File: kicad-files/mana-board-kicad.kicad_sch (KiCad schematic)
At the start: 39 parts, among them U1 Pico

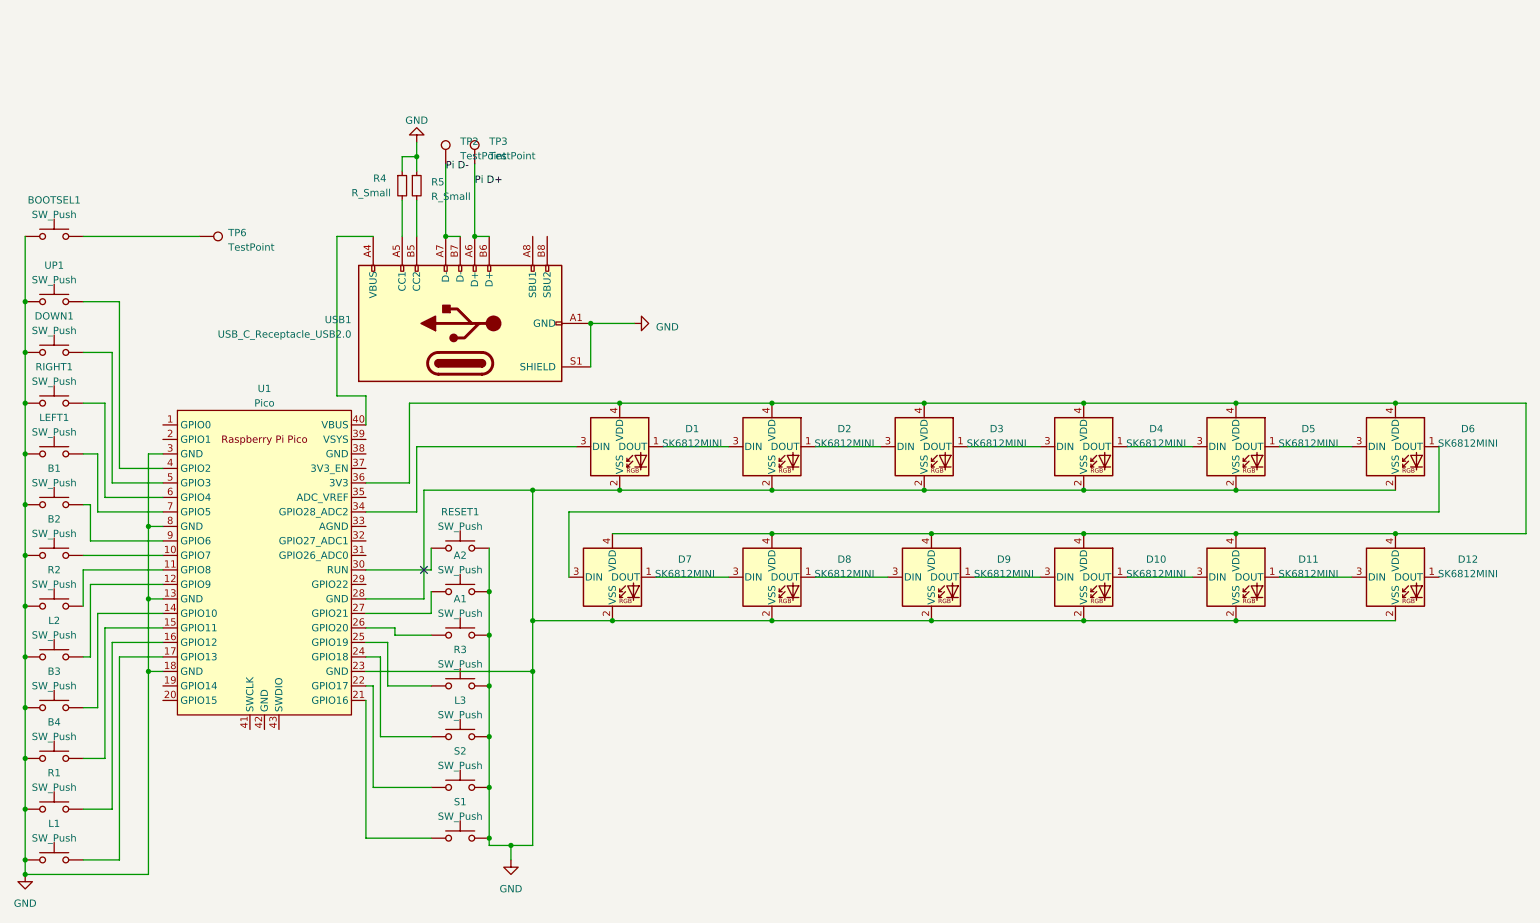
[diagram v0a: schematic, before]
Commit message: Organize libraries, start rev1
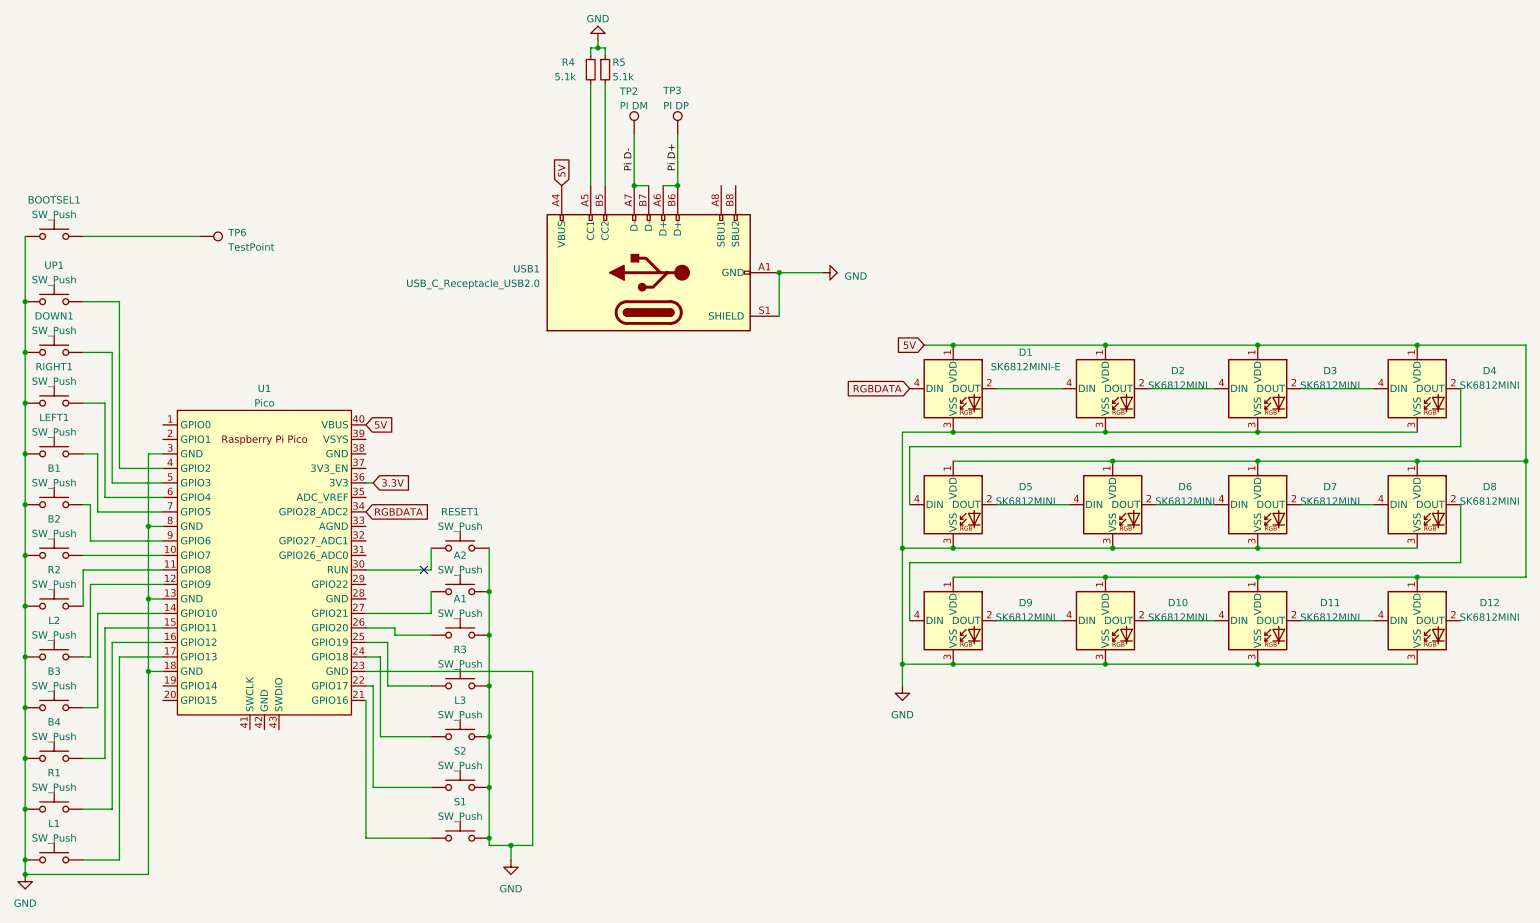
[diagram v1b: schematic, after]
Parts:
- D1: value SK6812MINI -> SK6812MINI-E; footprint Footprints:SK6812-MINI-E-reversed -> Keebio-Parts:SK6812-MINI-E; symbol LED:SK6812MINI -> ManaBoard:SK6812MINI-E
- D10, D11, D12, D2, D3, D4, D5, D6, D7, D8, D9: footprint Footprints:SK6812-MINI-E-reversed -> Keebio-Parts:SK6812-MINI-E; symbol LED:SK6812MINI -> ManaBoard:SK6812MINI-E
- R4, R5: value R_Small -> 5.1k
- TP2: value TestPoint -> PI DM
- TP3: value TestPoint -> PI DP
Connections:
- net GND: now also D1.3 (VSS), D10.3 (VSS), D11.3 (VSS), D12.3 (VSS), D2.3 (VSS), D3.3 (VSS), D4.3 (VSS), D5.3 (VSS), D6.3 (VSS), D7.3 (VSS), D8.3 (VSS), D9.3 (VSS); no longer D1.2 (VSS), D10.2 (VSS), D11.2 (VSS), D12.2 (VSS), D2.2 (VSS), D3.2 (VSS), D4.2 (VSS), D5.2 (VSS), D6.2 (VSS), D7.2 (VSS), D8.2 (VSS), D9.2 (VSS), U1.28 (GND)
- net 5V: now reaches D4.1 (VDD)
- net 5V: now also D1.1 (VDD), D10.1 (VDD), D11.1 (VDD), D12.1 (VDD), D2.1 (VDD), D3.1 (VDD), D5.1 (VDD), D6.1 (VDD), D7.1 (VDD), D8.1 (VDD), D9.1 (VDD), U1.40 (VBUS), USB1.A4 (VBUS), USB1.A9 (VBUS), USB1.B4 (VBUS), USB1.B9 (VBUS); no longer D5.3 (DIN)
- net RGBDATA: now reaches U1.34 (GPIO28_ADC2)
- net RGBDATA: now also D1.4 (DIN); no longer D1.3 (DIN)
- new net: D4.2 (DOUT), D5.4 (DIN)
- new net: D3.2 (DOUT), D4.4 (DIN)
- new net: D2.2 (DOUT), D3.4 (DIN)
- new net: D5.2 (DOUT), D6.4 (DIN)
- new net: D11.2 (DOUT), D12.4 (DIN)
- new net: D10.2 (DOUT), D11.4 (DIN)
- new net: D7.2 (DOUT), D8.4 (DIN)
- new net: D6.2 (DOUT), D7.4 (DIN)
- new net: D10.4 (DIN), D9.2 (DOUT)
- new net: D8.2 (DOUT), D9.4 (DIN)
- new net: D1.2 (DOUT), D2.4 (DIN)
- new net 3.3V: U1.36 (3V3)
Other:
- moved on the sheet: D1, D10, D11, D12, D2, D3, D4, D5, D6, D7, D8, D9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
